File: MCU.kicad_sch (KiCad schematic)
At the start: 3 parts, among them U1 ESP32-S2-SOLO-N4

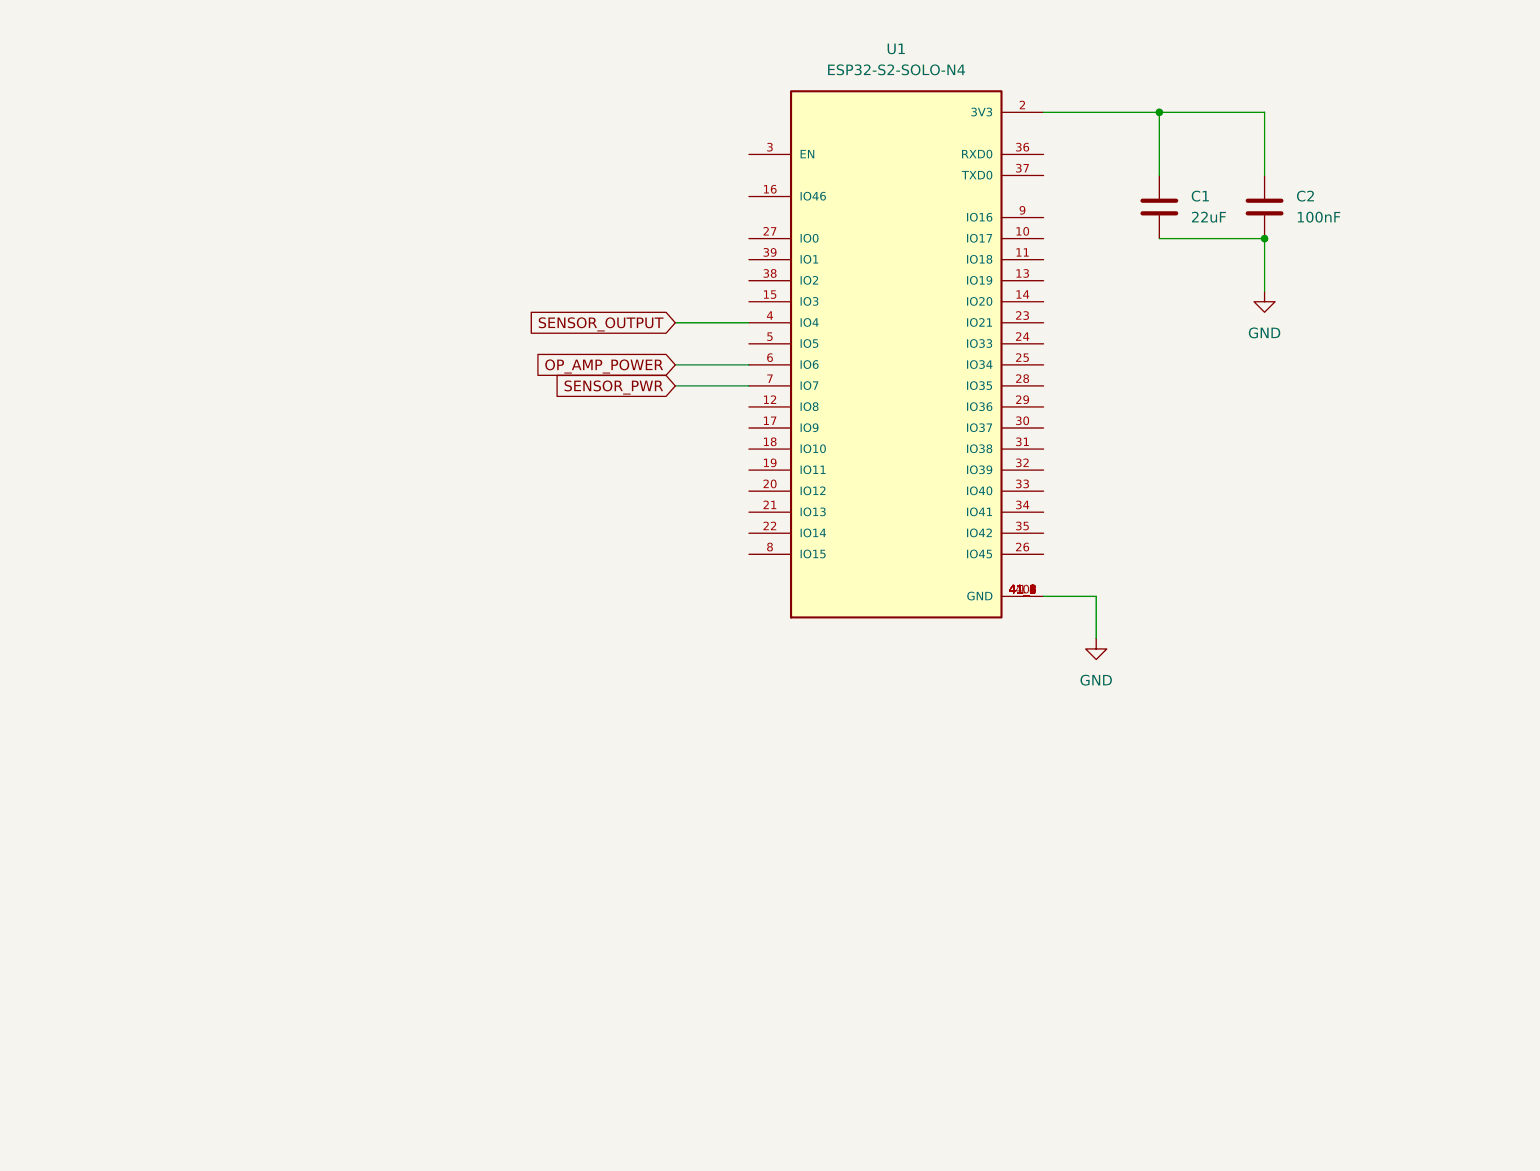
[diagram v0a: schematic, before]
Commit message: Completed first iteration and reviews
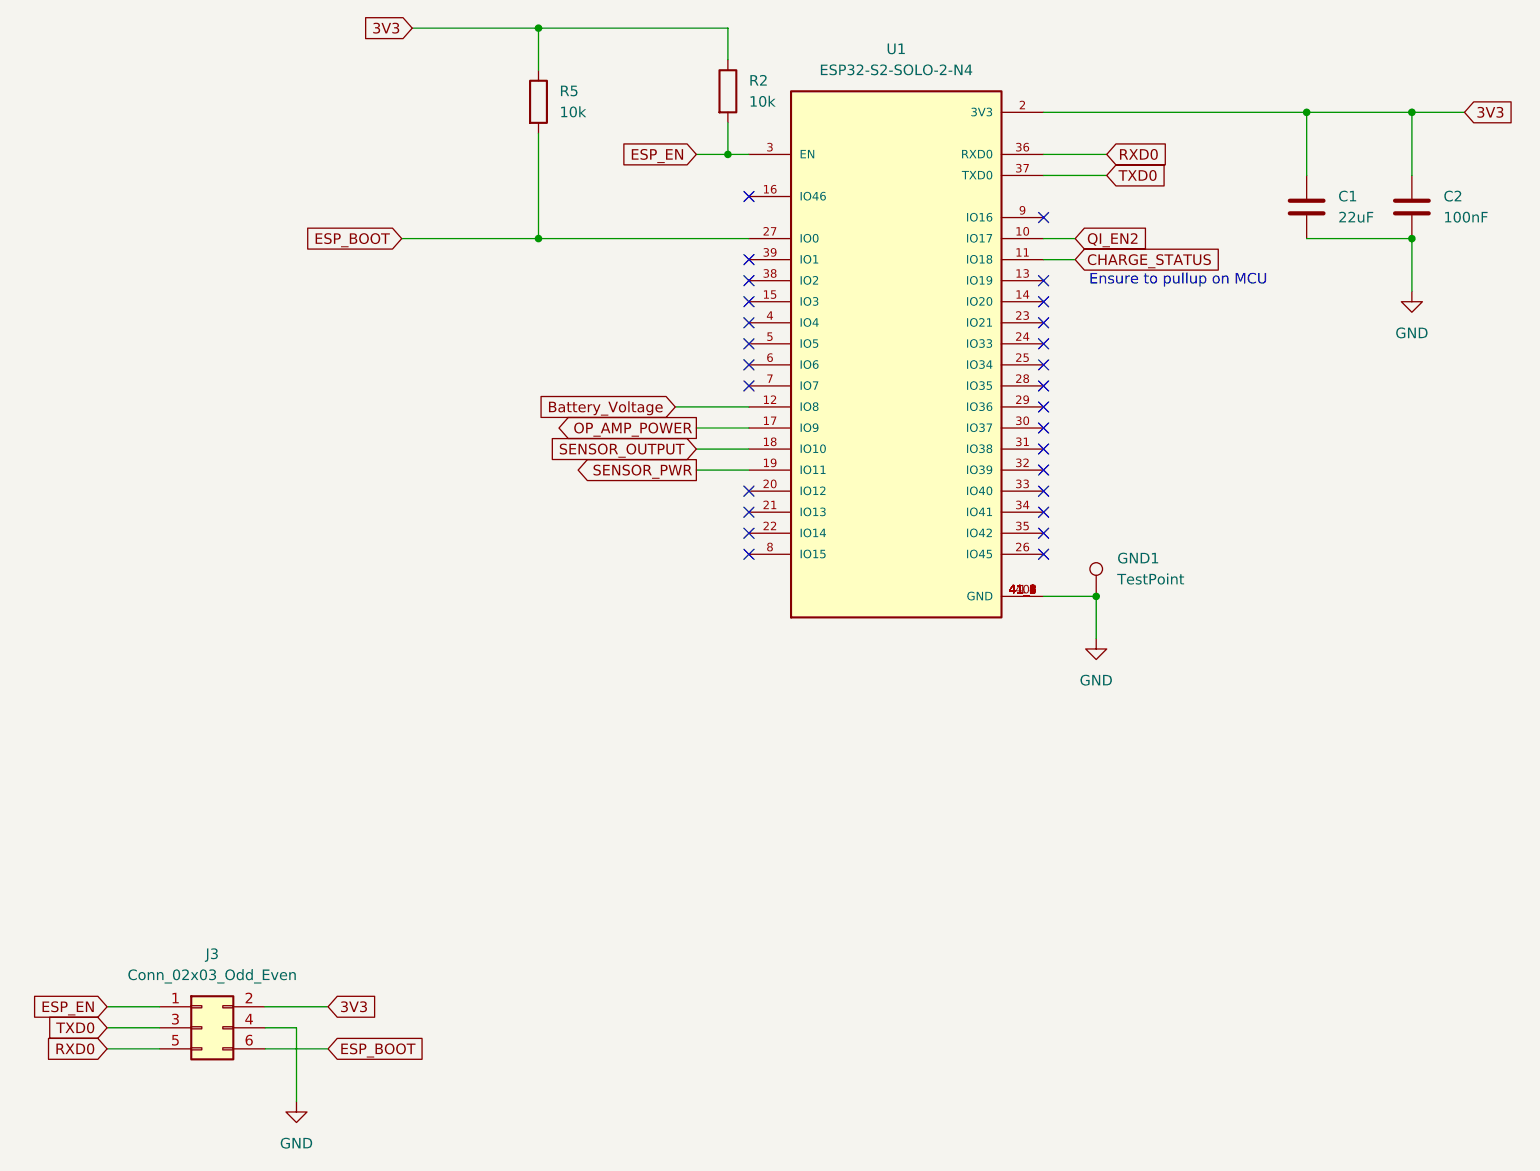
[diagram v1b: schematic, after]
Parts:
- added GND1: TestPoint, TestPoint:TestPoint_Pad_D1.0mm, symbol Connector:TestPoint
- added J3: Conn_02x03_Odd_Even, Connector_PinHeader_1.27mm:PinHeader_2x03_P1.27mm_Vertical_SMD, symbol Connector_Generic:Conn_02x03_Odd_Even
- added R2, R5: 10k, Resistor_SMD:R_0805_2012Metric_Pad1.20x1.40mm_HandSolder, symbol Device:R
- C1: footprint (none) -> Capacitor_SMD:C_0805_2012Metric_Pad1.18x1.45mm_HandSolder; Supplier (none) -> Digikey; Supplier Part Number (none) -> 1276-CL21A226MAYNNNECT-ND
- C2: footprint (none) -> Capacitor_SMD:C_0805_2012Metric_Pad1.18x1.45mm_HandSolder; Supplier (none) -> Digikey; Supplier Part Number (none) -> 1276-1003-1-ND
- U1: value ESP32-S2-SOLO-N4 -> ESP32-S2-SOLO-2-N4; footprint ESP32-S2-SOLO-N4:XCVR_ESP32-S2-SOLO-N4 -> Hydro_footprints:ESP32-S2-SOLO-N4; Supplier (none) -> Digikey; Supplier Part Number (none) -> 1965-ESP32-S2-SOLO-2-N4CT-ND
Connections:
- net GND: now also GND1.1, J3.4 (Pin_4)
- net OP_AMP_POWER: now also U1.17 (IO9); no longer U1.6 (IO6)
- net SENSOR_OUTPUT: now also U1.18 (IO10); no longer U1.4 (IO4)
- net SENSOR_PWR: now also U1.19 (IO11); no longer U1.7 (IO7)
- net 3V3: now reaches C1.1, C2.1, U1.2 (3V3)
- net 3V3: now also J3.2 (Pin_2), R2.1, R5.1
- net QI_EN2: now reaches U1.10 (IO17)
- net CHARGE_STATUS: now reaches U1.11 (IO18)
- net Battery_Voltage: now reaches U1.12 (IO8)
- net ESP_BOOT: now reaches U1.27 (IO0)
- net ESP_BOOT: now also J3.6 (Pin_6), R5.2
- net ESP_EN: now reaches U1.3 (EN)
- net ESP_EN: now also J3.1 (Pin_1), R2.2
- net RXD0: now reaches U1.36 (RXD0)
- net RXD0: now also J3.5 (Pin_5)
- net TXD0: now reaches U1.37 (TXD0)
- net TXD0: now also J3.3 (Pin_3)
- no-connect marks 0 -> 27
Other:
- note added: "Ensure to pullup on MCU"
- company: (none) -> Horatio Pistachio
- title: (none) -> WashingLineMonitor-P0001
- moved on the sheet: C1, C2

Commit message: commit of local files before designing next version
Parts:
- J3: Digikey_Part_Number (none) -> SAM13920TR-ND; Part_Number SAM13920TR-ND -> (none)
- U1: JLC_Part_Number (none) -> C3040594
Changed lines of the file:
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@@
+			)
+		)
+		(property "JLC_Part_Number" ""
+			(at 175.26 77.47 0)
+			(effects
+				(font
+					(size 1.27 1.27)
+				)
+				(hide yes)
 			)
 		)
@@
 			)
 		)
-		(property "Part_Number" "SAM13920TR-ND"
-			(at 41.91 176.53 0)
-			(effects
-				(font
-					(size 1.27 1.27)
-				)
-				(hide yes)
-			)
-		)
 		(property "Supplier" "Digikey"
 			(at 41.91 176.53 0)
@@
 		)
 		(property "Supplier Part Number" "SAM13920TR-ND"
+			(at 41.91 176.53 0)
+			(effects
+				(font
+					(size 1.27 1.27)
+				)
+				(hide yes)
+			)
+		)
+		(property "Digikey_Part_Number" "SAM13920TR-ND"
+			(at 41.91 176.53 0)
+			(effects
+				(font
+					(size 1.27 1.27)
+				)
+				(hide yes)
+			)
+		)
+		(property "JLC_Part_Number" ""
 			(at 41.91 176.53 0)
 			(effects
@@
 			)
 		)
+		(property "JLC_Part_Number" ""
+			(at 105.41 63.5 0)
+			(effects
+				(font
+					(size 1.27 1.27)
+				)
+				(hide yes)
+			)
+		)
 		(pin "1"
 		)
@@
 			)
 		)
+		(property "JLC_Part_Number" "C3040594"
+			(at 125.73 96.52 0)
+			(effects
+				(font
+					(size 1.27 1.27)
+				)
+				(hide yes)
+			)
+		)
 		(pin "38"
 		)
@@
 			)
 		)
+		(property "JLC_Part_Number" ""
+			(at 82.55 64.77 0)
+			(effects
+				(font
+					(size 1.27 1.27)
+				)
+				(hide yes)
+			)
+		)
 		(pin "1"
 		)
@@
 			)
 		)
+		(property "JLC_Part_Number" ""
+			(at 149.86 124.46 0)
+			(effects
+				(font
+					(size 1.27 1.27)
+				)
+				(hide yes)
+			)
+		)
 		(pin "1"
 		)
@@
 			(at 187.96 77.47 0)
 			(effects
+				(font
+					(size 1.27 1.27)
+				)
+				(hide yes)
+			)
+		)
+		(property "JLC_Part_Number" ""
+			(at 187.96 77.47 0)
+			(effects
